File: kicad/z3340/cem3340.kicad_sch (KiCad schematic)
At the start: 63 parts, among them Q1 2N7002, Q2 2N7002, U1 DG442CY+, U2 AS3340, U3 LM79L05, U4 LM311, U5 TL074, U7 LM4040B-5, U8 DG442CY+

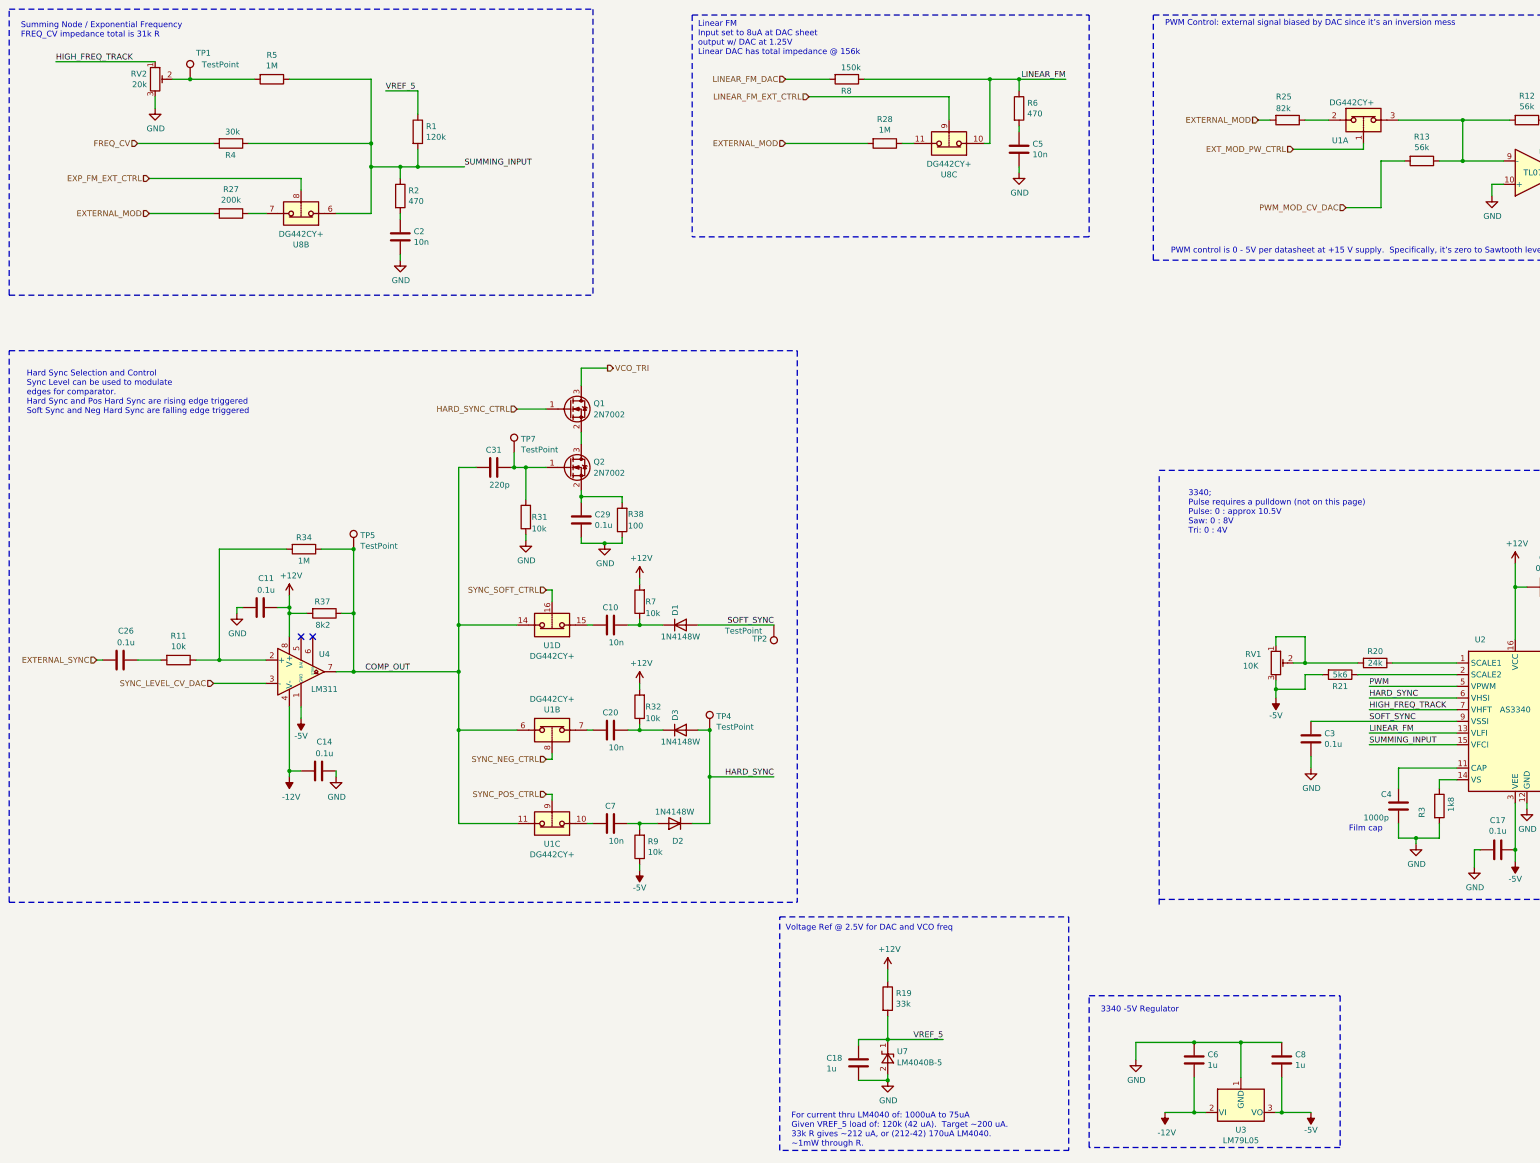
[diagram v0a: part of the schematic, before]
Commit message: cleaning up and rename dir to z3340
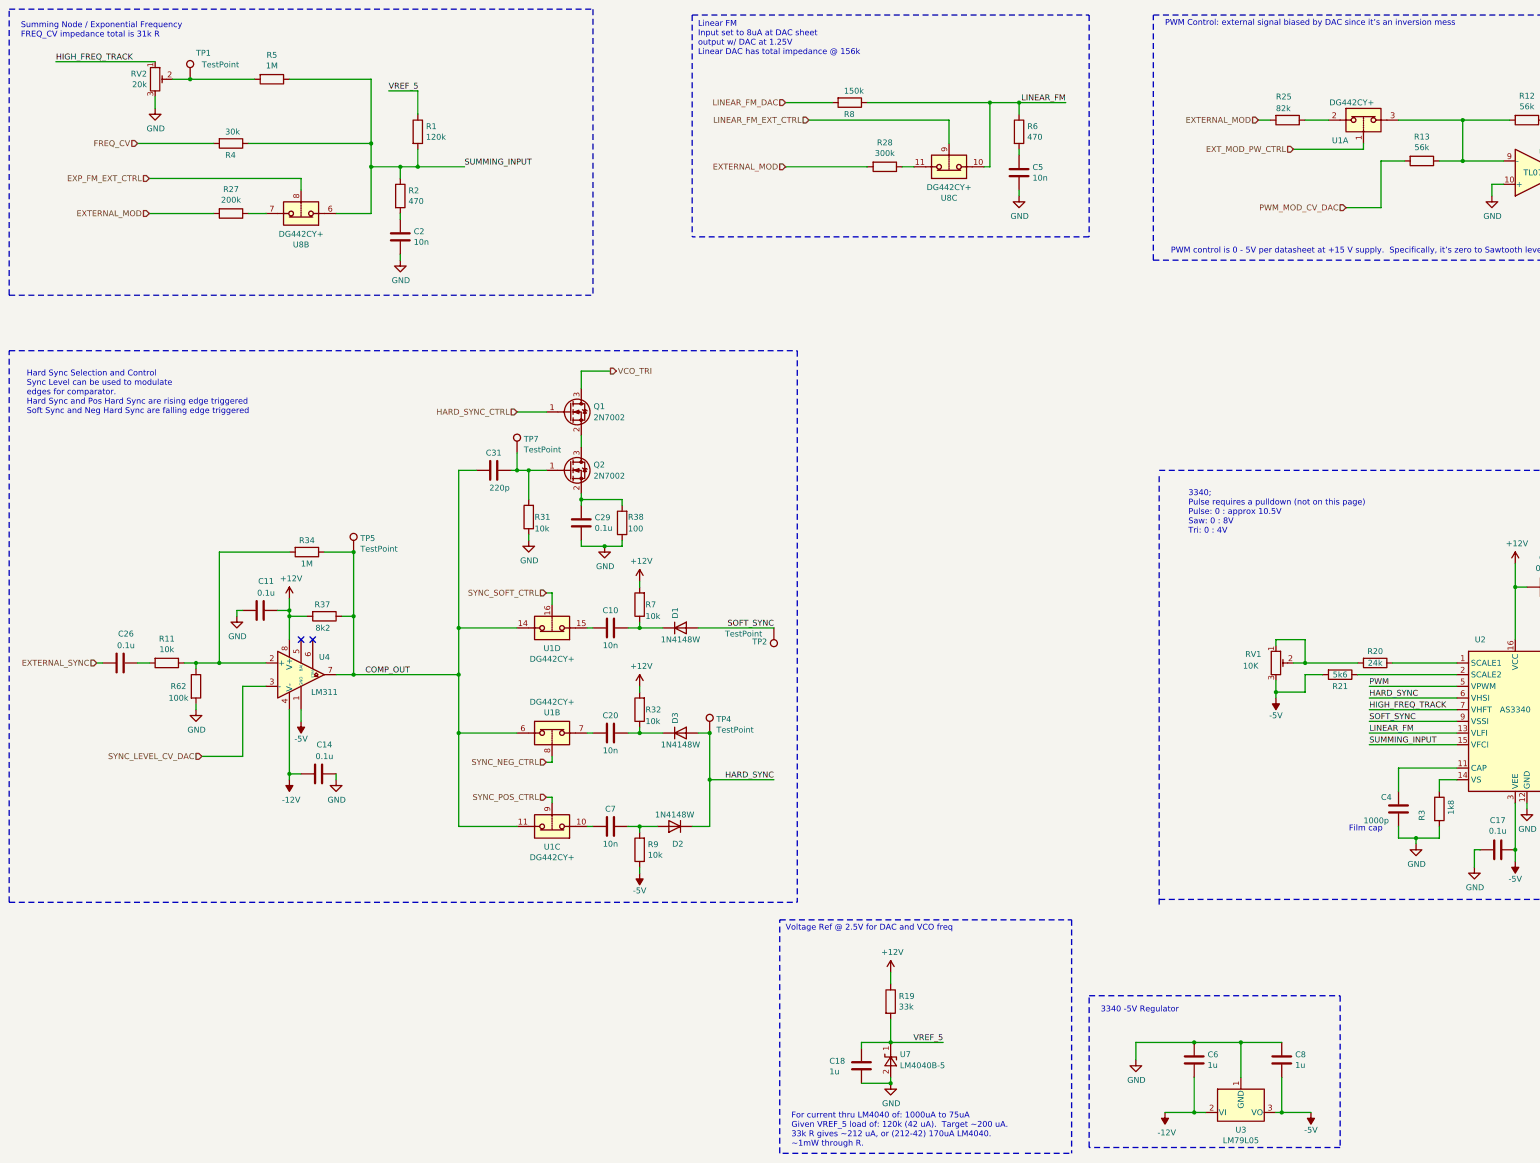
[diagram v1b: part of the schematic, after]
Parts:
- removed C3: 0.1u, Capacitor_SMD:C_0603_1608Metric, symbol Device:C
- added R62: 100k, Resistor_SMD:R_0603_1608Metric, symbol Device:R
- R28: value 1M -> 300k; LCSC Part C22935 -> (none)
- R37: footprint Resistor_SMD:R_0603_1608Metric -> Resistor_SMD:R_0805_2012Metric; LCSC Part C25981 -> C17828
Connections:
- net GND: now also R62.2
- net at R11.1, R34.2, U4.2 (+): now also R62.1
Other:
- moved on the sheet: C10, C11, C14, C18, C20, C26, C29, C31, C4, C5, C7, D1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
